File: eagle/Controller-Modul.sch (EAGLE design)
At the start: 36 parts, among them IC3 ATMEGA328P, Q1 BC550C

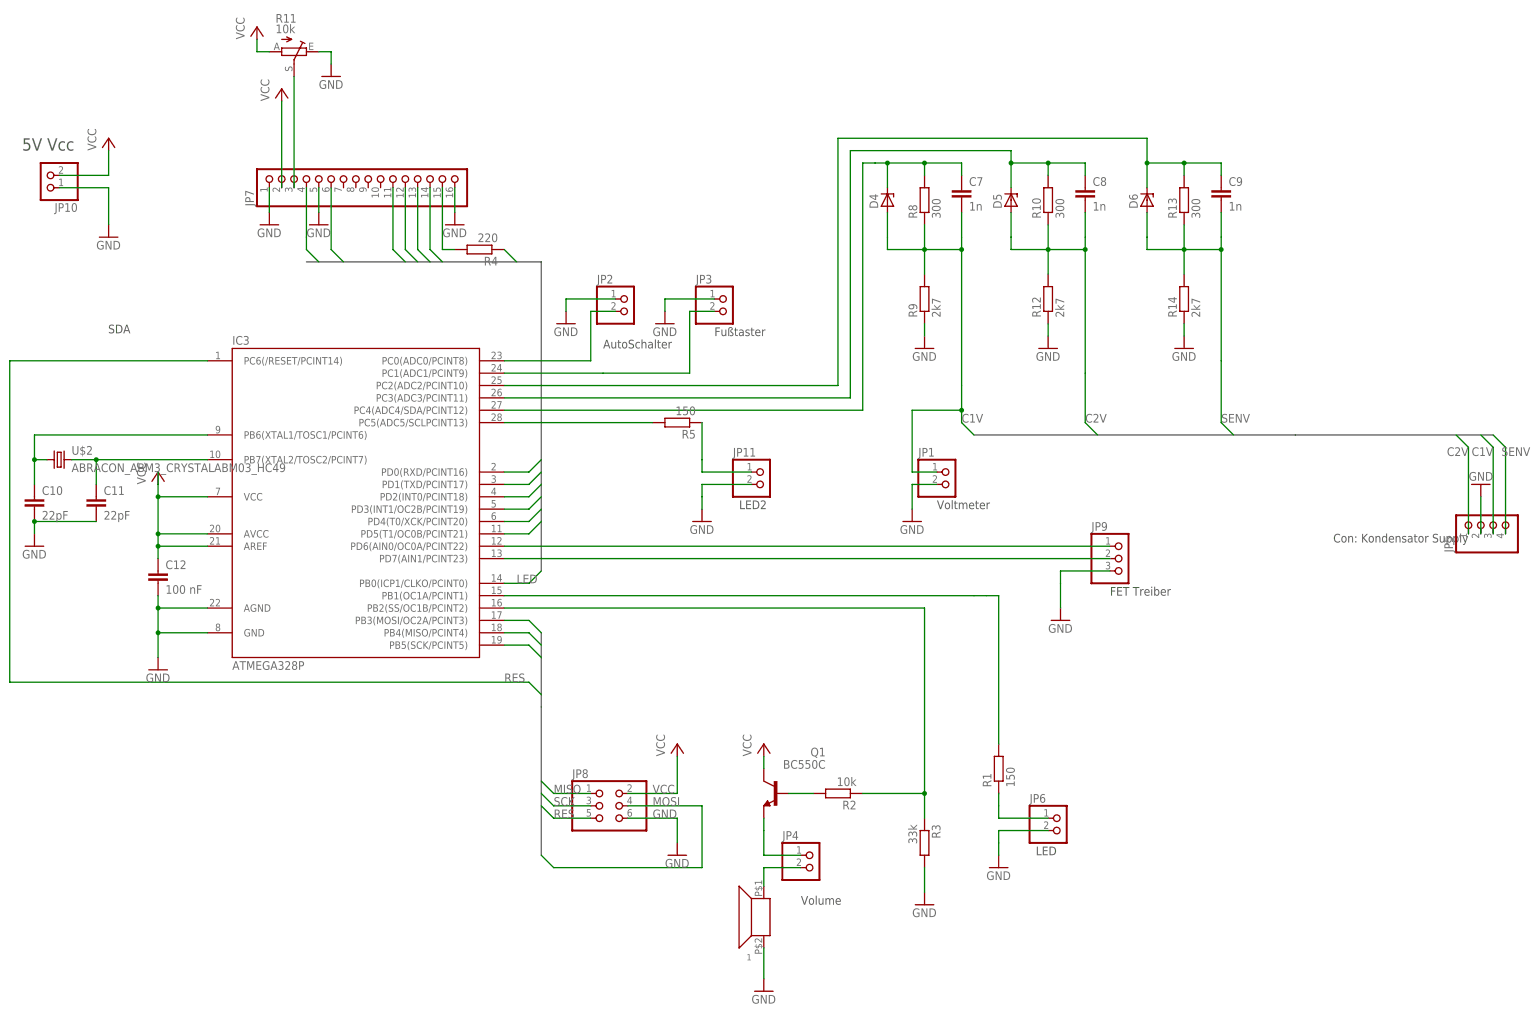
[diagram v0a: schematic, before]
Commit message: Var. Changes. Layout and new diode for 7818
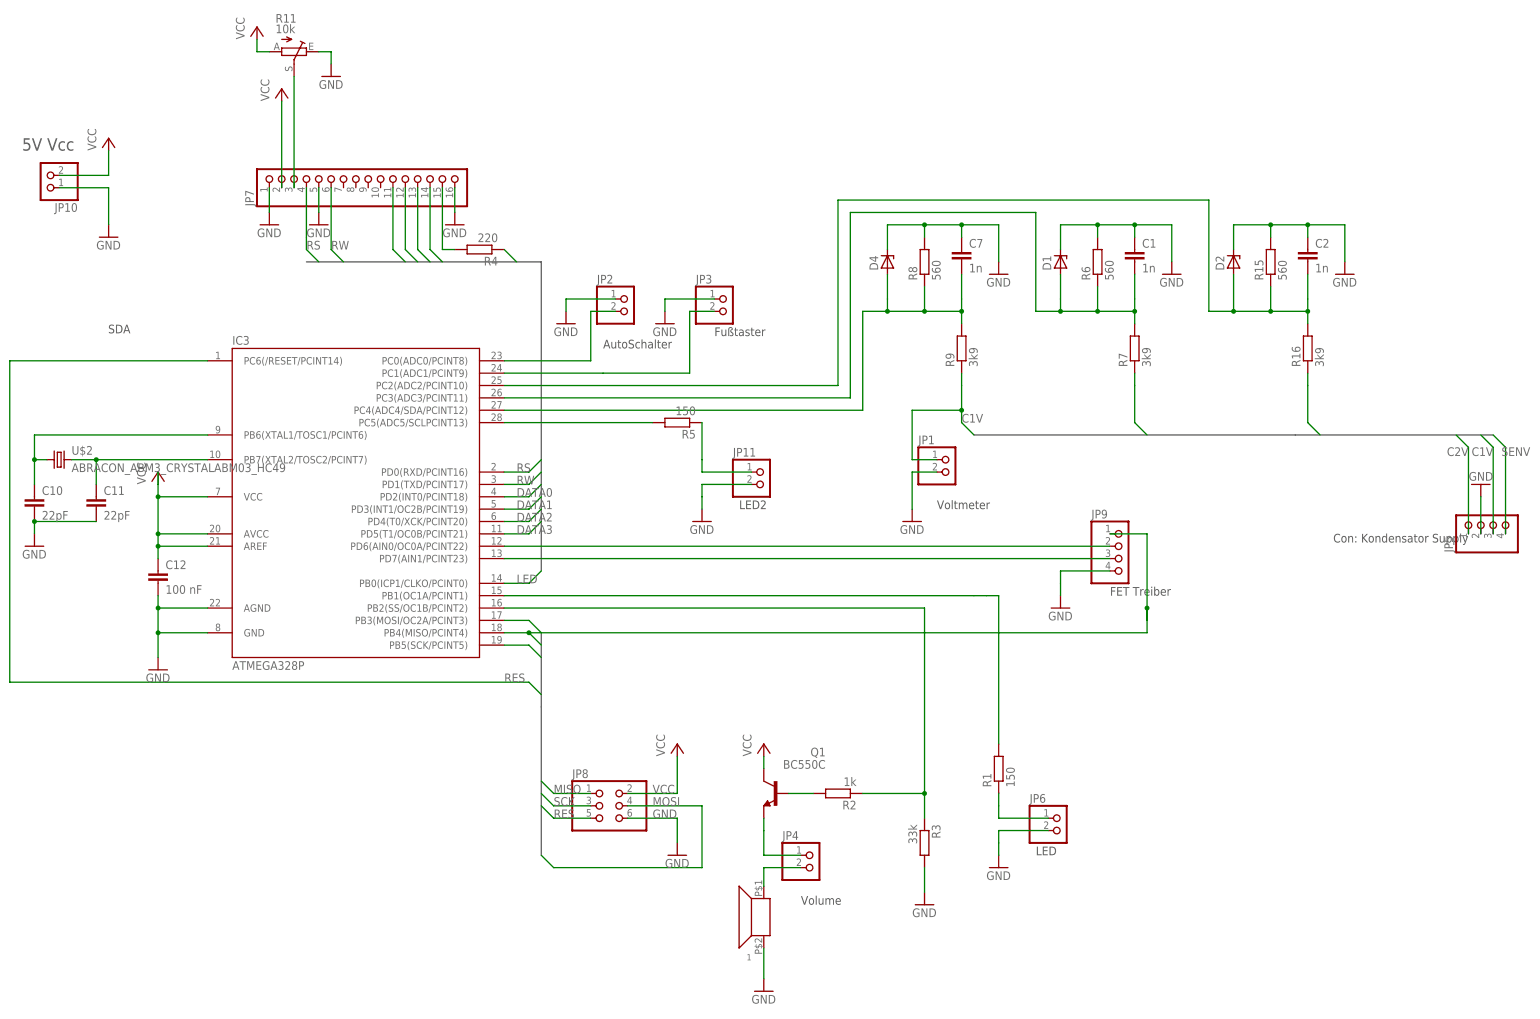
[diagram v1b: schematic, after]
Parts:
- removed C8, C9: 1n, rcl:C-EUC0603K
- removed D5, D6: (no value), diode:ZENER-DIODESOT23
- removed R10, R13: 300, resistor:R-EU_R1206
- removed R12, R14: 2k7, resistor:R-EU_R1206
- added C1, C2: 1n, rcl:C-EUC0603K
- added D1, D2: (no value), diode:ZENER-DIODESOT23
- added R15, R6: 560, resistor:R-EU_R1206
- added R16, R7: 3k9, resistor:R-EU_R1206
- JP9: device pinhead:PINHD-1X3 -> pinhead:PINHD-1X4
- R2: value 10k -> 1k
- R8: value 300 -> 560
- R9: value 2k7 -> 3k9
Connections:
- removed net N$14: C7.1, D4.C, IC3.PC4(ADC4/SDA/PCINT12), R8.2
- removed net N$24: C8.1, D5.C, IC3.PC3(ADC3/PCINT11), R10.2
- new net N$5: C7.2, D4.A, IC3.PC4(ADC4/SDA/PCINT12), R8.1, R9.2
- new net N$7: C1.2, D1.A, IC3.PC3(ADC3/PCINT11), R6.1, R7.2
- net C1V: now also R9.1; no longer C7.2, D4.A, R8.1, R9.2
- net C2V: now also R7.1; no longer C8.2, D5.A, R10.1, R12.2
- net GND: now also C1.1, C2.1, C7.1, D1.C, D2.C, D4.C, JP9.4, R15.2, R6.2, R8.2; no longer JP9.3, R12.1, R14.1, R9.1
- net MISO: now also JP9.1
- net N$18: now also C2.2, D2.A, R15.1, R16.2; no longer C9.1, D6.C, R13.2
- net N$31: now also JP9.3; no longer JP9.2
- net N$34: now also JP9.2; no longer JP9.1
- net SENV: now also R16.1; no longer C9.2, D6.A, R13.1, R14.2
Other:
- moved on the sheet: C7, D4, JP1, R8, R9
